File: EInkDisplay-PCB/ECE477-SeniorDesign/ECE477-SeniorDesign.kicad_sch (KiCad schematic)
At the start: 1 part

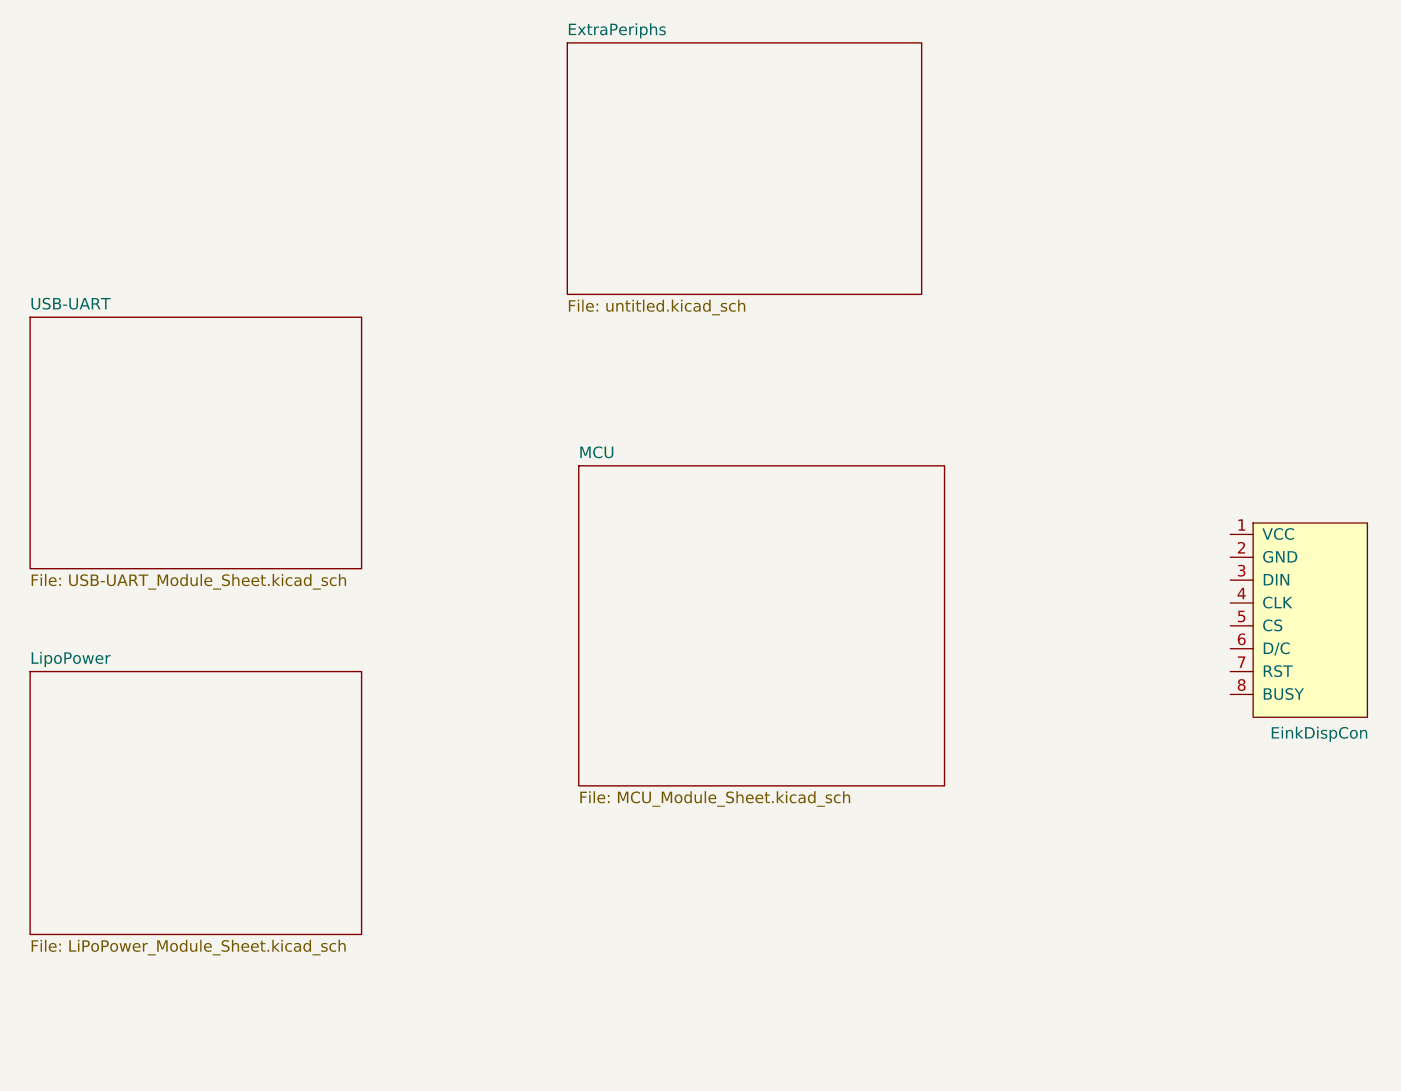
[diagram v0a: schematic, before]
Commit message: push
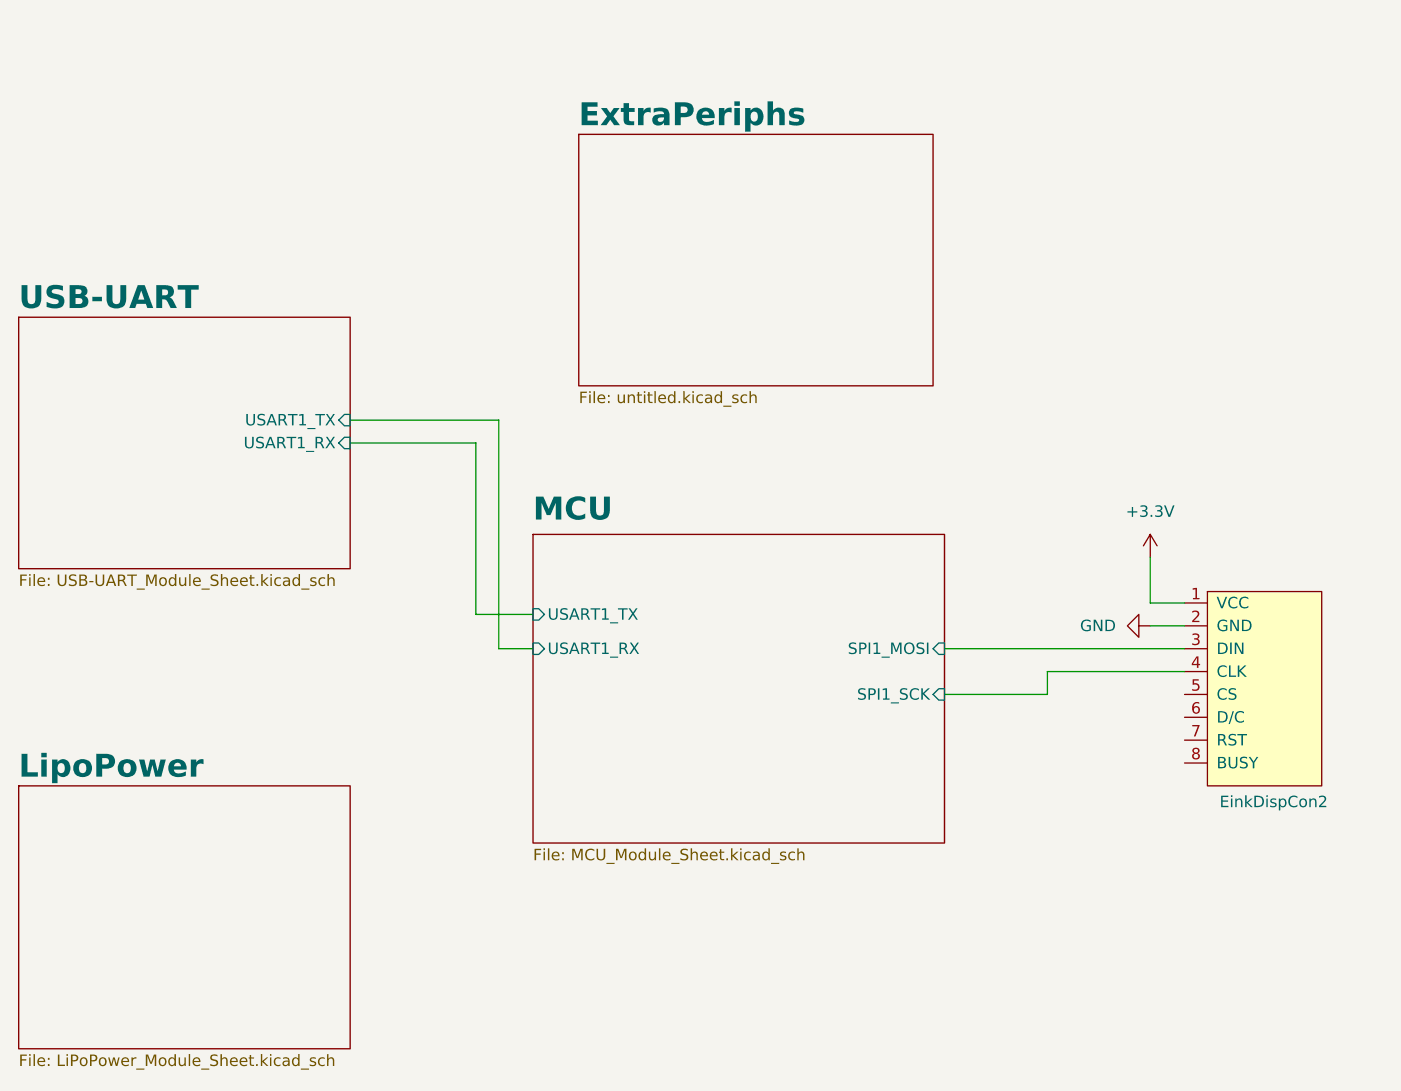
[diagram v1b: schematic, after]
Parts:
- removed EinkDispCon: ~, symbol EinkComponentLibrary:EinkDisplay
- added EinkDispCon2: ~, symbol EinkComponentLibrary:EinkDisplay
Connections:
- new net +3.3V: EinkDispCon2.1 (VCC)
- new net GND: EinkDispCon2.2 (GND)
- new net MCU/SPI1_MOSI: EinkDispCon2.3 (DIN)
- new net MCU/SPI1_SCK: EinkDispCon2.4 (CLK)
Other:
- sheet MCU ports: added SPI1_MOSI, SPI1_SCK, USART1_RX, USART1_TX; removed none
- sheet USB-UART ports: added USART1_RX, USART1_TX; removed none
